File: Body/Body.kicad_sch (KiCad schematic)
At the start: 32 parts, among them J1 Arduino_Nano_Header, J2 TB_1X2, J3 Cable_PAD, J4 TB_1X2, J5 TB_1X2, J6 Cable_PAD, J7 CONN_01X10, J8 Cable_PAD, J9 Cable_PAD, SW1 SW_SPDT, SW4 SW_Push, SW5 SW_Push, U1 DRV8833_MODULE, U2 LM78XX, U3 DRV8833_MODULE

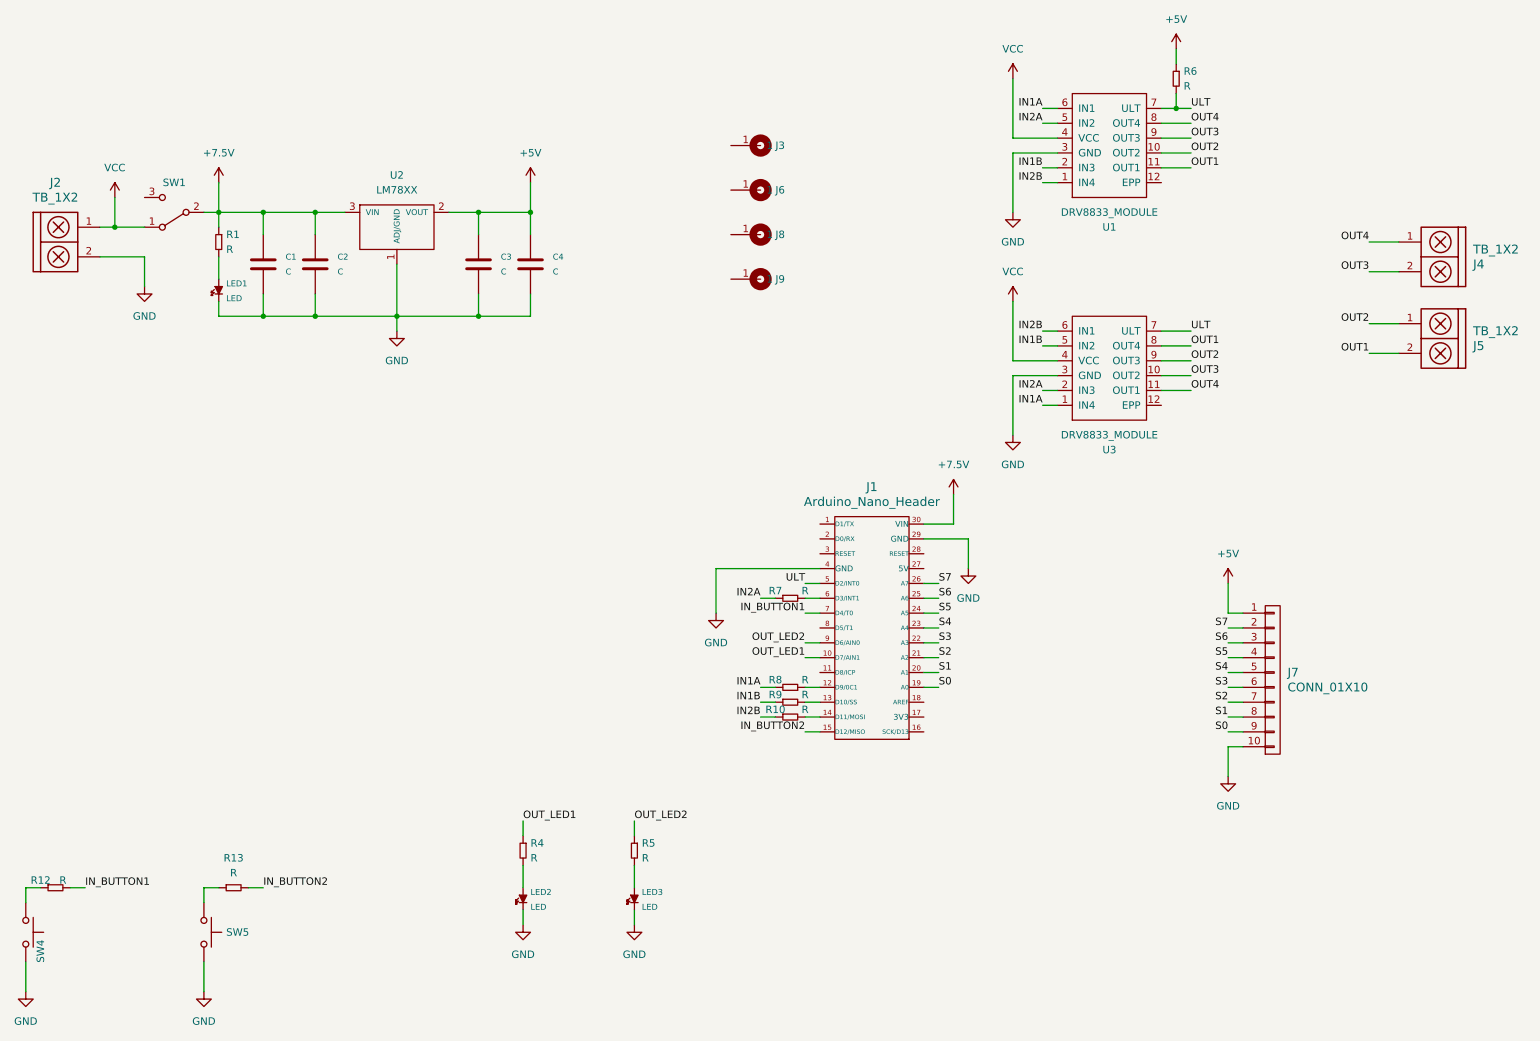
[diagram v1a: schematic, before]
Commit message: Rev 1.0.1
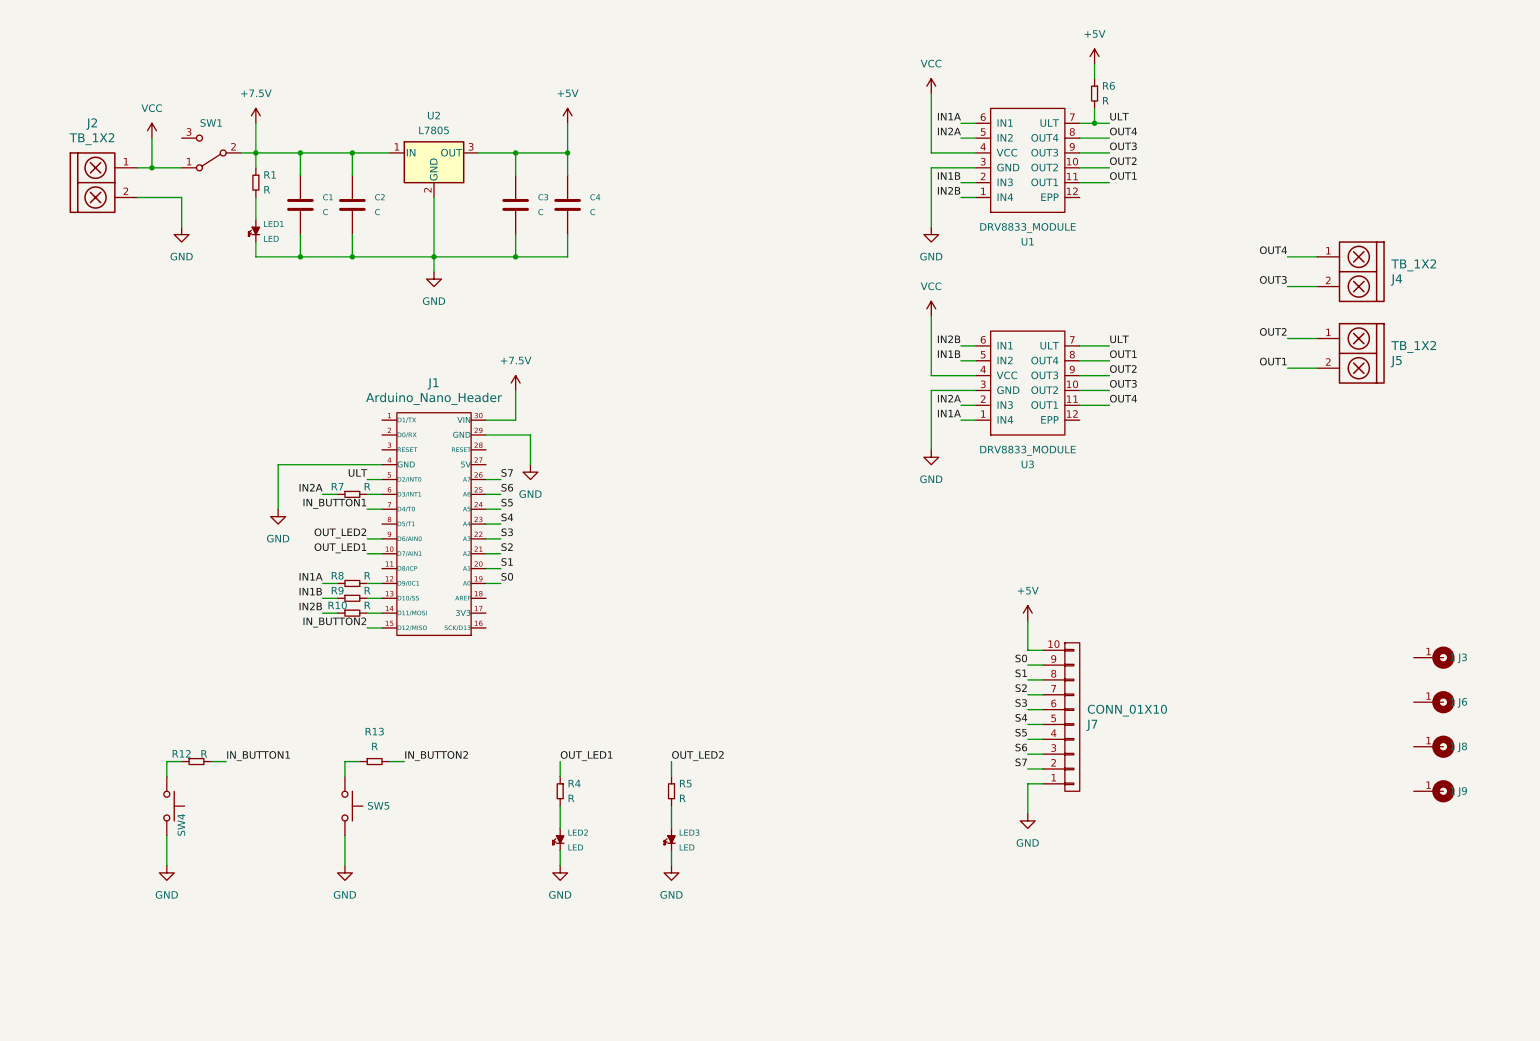
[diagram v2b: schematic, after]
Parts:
- removed U2: LM78XX, MacroLib:TO-220-3_Vertical, symbol MacroLib:LM78XX
- added U2: L7805, MacroLib:TO-220-3_Vertical, symbol Regulator_Linear:L7805
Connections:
- net +5V: now also J7.10, U2.3 (OUT); no longer J7.1
- net +7.5V: now also U2.1 (IN)
- net GND: now also J7.1, U2.2 (GND); no longer J7.10
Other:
- moved on the sheet: C1, C2, C3, C4, J1, J2, J3, J4, J5, J6, J7, J8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
